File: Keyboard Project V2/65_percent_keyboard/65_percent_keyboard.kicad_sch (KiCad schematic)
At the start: 5 parts, among them U1 ATmega32A-P, Y1 16MHz

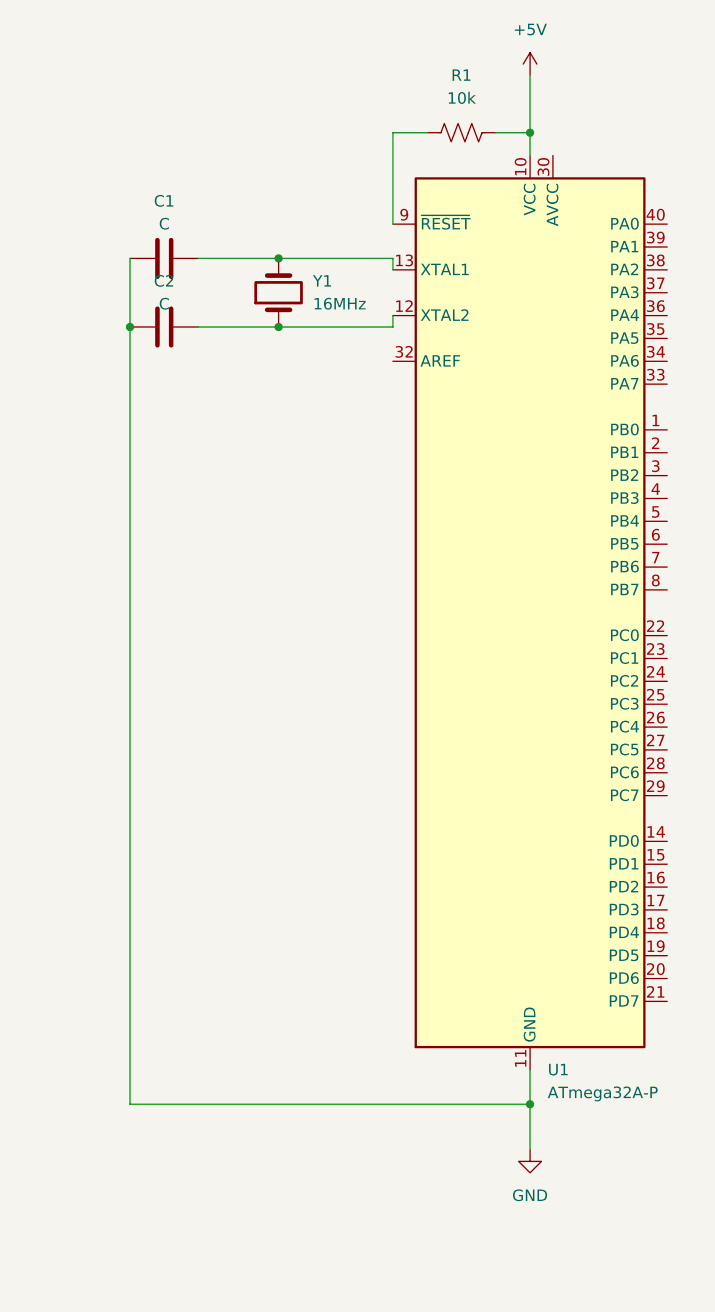
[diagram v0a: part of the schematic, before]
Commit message: updated directory
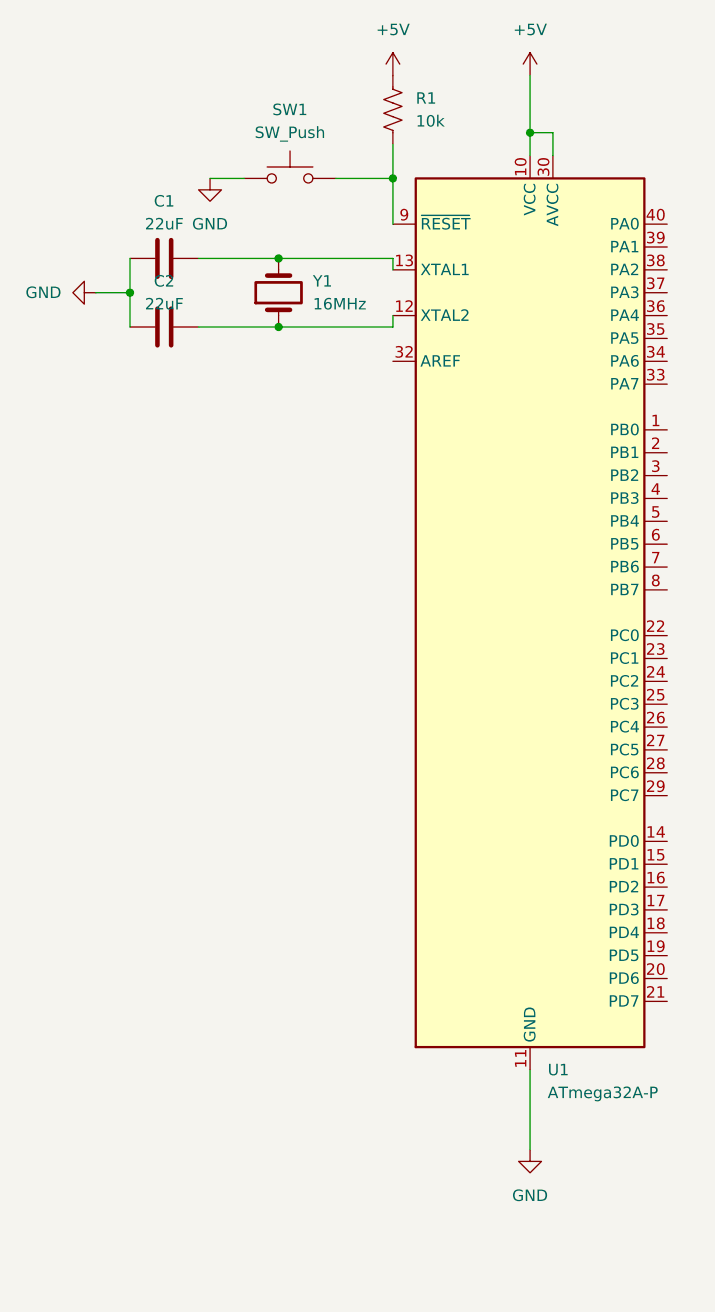
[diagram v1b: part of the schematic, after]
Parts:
- added SW1: SW_Push, symbol Switch:SW_Push
- C1, C2: value C -> 22uF
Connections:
- net +5V: now also U1.30 (AVCC)
- net GND: now also SW1.1
- net at R1.1, U1.9 (~{RESET}): now also SW1.2
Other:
- moved on the sheet: R1
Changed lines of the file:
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@@
 (kicad_sch (version 20230121) (generator eeschema)
   (paper "A4")
-  (junction (at 66.04 143.51) (diameter 0) (color 0 0 0 0)
+  (junction (at 50.8 40.64) (diameter 0) (color 0 0 0 0)
+  )
+  (junction (at 21.59 53.34) (diameter 0) (color 0 0 0 0)
   )
   (junction (at 38.1 57.15) (diameter 0) (color 0 0 0 0)
@@
   (junction (at 66.04 35.56) (diameter 0) (color 0 0 0 0)
   )
-  (junction (at 21.59 57.15) (diameter 0) (color 0 0 0 0)
-  )
   (junction (at 38.1 49.53) (diameter 0) (color 0 0 0 0)
   )
-  (wire (pts (xy 21.59 49.53) (xy 21.59 57.15))
-    (stroke (width 0) (type default))
-  )
-  (wire (pts (xy 66.04 143.51) (xy 21.59 143.51))
-    (stroke (width 0) (type default))
-  )
-  (wire (pts (xy 50.8 45.72) (xy 50.8 35.56))
-    (stroke (width 0) (type default))
-  )
-  (wire (pts (xy 62.23 35.56) (xy 66.04 35.56))
-    (stroke (width 0) (type default))
-  )
-  (wire (pts (xy 50.8 35.56) (xy 54.61 35.56))
-    (stroke (width 0) (type default))
-  )
-  (wire (pts (xy 66.04 139.7) (xy 66.04 143.51))
+  (wire (pts (xy 68.58 35.56) (xy 68.58 38.1))
+    (stroke (width 0) (type default))
+  )
+  (wire (pts (xy 21.59 49.53) (xy 21.59 53.34))
+    (stroke (width 0) (type default))
+  )
+  (wire (pts (xy 50.8 40.64) (xy 50.8 45.72))
+    (stroke (width 0) (type default))
+  )
+  (wire (pts (xy 17.78 53.34) (xy 21.59 53.34))
+    (stroke (width 0) (type default))
+  )
+  (wire (pts (xy 21.59 53.34) (xy 21.59 57.15))
+    (stroke (width 0) (type default))
+  )
+  (wire (pts (xy 66.04 35.56) (xy 68.58 35.56))
     (stroke (width 0) (type default))
   )
@@
     (stroke (width 0) (type default))
   )
+  (wire (pts (xy 44.45 40.64) (xy 50.8 40.64))
+    (stroke (width 0) (type default))
+  )
   (wire (pts (xy 66.04 35.56) (xy 66.04 38.1))
     (stroke (width 0) (type default))
   )
+  (wire (pts (xy 50.8 36.83) (xy 50.8 40.64))
+    (stroke (width 0) (type default))
+  )
   (wire (pts (xy 38.1 49.53) (xy 50.8 49.53))
     (stroke (width 0) (type default))
   )
-  (wire (pts (xy 66.04 143.51) (xy 66.04 148.59))
-    (stroke (width 0) (type default))
-  )
-  (wire (pts (xy 21.59 143.51) (xy 21.59 57.15))
+  (wire (pts (xy 66.04 139.7) (xy 66.04 148.59))
     (stroke (width 0) (type default))
   )
   (wire (pts (xy 66.04 29.21) (xy 66.04 35.56))
+    (stroke (width 0) (type default))
+  )
+  (wire (pts (xy 34.29 40.64) (xy 30.48 40.64))
     (stroke (width 0) (type default))
   )
@@
         (path "/317806f0-7832-447d-a362-c03f416f1932"
           (reference "Y1") (unit 1)
+        )
+      )
+    )
+  )
+  (symbol (lib_id "power:GND") (at 30.48 40.64 0) (unit 1)
+    (in_bom yes) (on_board yes) (dnp no) (fields_autoplaced)
+    (property "Reference" "#PWR05" (at 30.48 46.99 0)
+      (effects (font (size 1.27 1.27)) hide)
+    )
+    (property "Value" "GND" (at 30.48 45.72 0)
+      (effects (font (size 1.27 1.27)))
+    )
+    (property "Footprint" "" (at 30.48 40.64 0)
+      (effects (font (size 1.27 1.27)) hide)
+    )
+    (property "Datasheet" "" (at 30.48 40.64 0)
+      (effects (font (size 1.27 1.27)) hide)
+    )
+    (pin "1")
+    (instances
+      (project "65_percent_keyboard"
+        (path "/317806f0-7832-447d-a362-c03f416f1932"
+          (reference "#PWR05") (unit 1)
         )
       )
@@
       (effects (font (size 1.27 1.27)))
     )
-    (property "Value" "C" (at 25.4 54.61 90)
+    (property "Value" "22uF" (at 25.4 54.61 90)
       (effects (font (size 1.27 1.27)))
     )
@@
         (path "/317806f0-7832-447d-a362-c03f416f1932"
           (reference "C2") (unit 1)
+        )
+      )
+    )
+  )
+  (symbol (lib_id "Switch:SW_Push") (at 39.37 40.64 0) (unit 1)
+    (in_bom yes) (on_board yes) (dnp no) (fields_autoplaced)
+    (property "Reference" "SW1" (at 39.37 33.02 0)
+      (effects (font (size 1.27 1.27)))
+    )
+    (property "Value" "SW_Push" (at 39.37 35.56 0)
+      (effects (font (size 1.27 1.27)))
+    )
+    (property "Footprint" "" (at 39.37 35.56 0)
+      (effects (font (size 1.27 1.27)) hide)
+    )
+    (property "Datasheet" "~" (at 39.37 35.56 0)
+      (effects (font (size 1.27 1.27)) hide)
+    )
+    (pin "1")
+    (pin "2")
+    (instances
+      (project "65_percent_keyboard"
+        (path "/317806f0-7832-447d-a362-c03f416f1932"
+          (reference "SW1") (unit 1)
+        )
+      )
+    )
+  )
+  (symbol (lib_id "power:GND") (at 17.78 53.34 270) (unit 1)
+    (in_bom yes) (on_board yes) (dnp no) (fields_autoplaced)
+    (property "Reference" "#PWR03" (at 11.43 53.34 0)
+      (effects (font (size 1.27 1.27)) hide)
+    )
+    (property "Value" "GND" (at 13.97 53.34 90)
+      (effects (font (size 1.27 1.27)) (justify right))
+    )
+    (property "Footprint" "" (at 17.78 53.34 0)
+      (effects (font (size 1.27 1.27)) hide)
+    )
+    (property "Datasheet" "" (at 17.78 53.34 0)
+      (effects (font (size 1.27 1.27)) hide)
+    )
+    (pin "1")
+    (instances
+      (project "65_percent_keyboard"
+        (path "/317806f0-7832-447d-a362-c03f416f1932"
+          (reference "#PWR03") (unit 1)
         )
       )
@@
       (effects (font (size 1.27 1.27)))
     )
-    (property "Value" "C" (at 25.4 45.72 90)
+    (property "Value" "22uF" (at 25.4 45.72 90)
       (effects (font (size 1.27 1.27)))
     )
@@
     )
   )
+  (symbol (lib_id "power:+5V") (at 50.8 29.21 0) (unit 1)
+    (in_bom yes) (on_board yes) (dnp no) (fields_autoplaced)
+    (property "Reference" "#PWR04" (at 50.8 33.02 0)
+      (effects (font (size 1.27 1.27)) hide)
+    )
+    (property "Value" "+5V" (at 50.8 24.13 0)
+      (effects (font (size 1.27 1.27)))
+    )
+    (property "Footprint" "" (at 50.8 29.21 0)
+      (effects (font (size 1.27 1.27)) hide)
+    )
+    (property "Datasheet" "" (at 50.8 29.21 0)
+      (effects (font (size 1.27 1.27)) hide)
+    )
+    (pin "1")
+    (instances
+      (project "65_percent_keyboard"
+        (path "/317806f0-7832-447d-a362-c03f416f1932"
+          (reference "#PWR04") (unit 1)
+        )
+      )
+    )
+  )
   (symbol (lib_id "power:GND") (at 66.04 148.59 0) (unit 1)
     (in_bom yes) (on_board yes) (dnp no) (fields_autoplaced)
@@
     )
   )
-  (symbol (lib_id "Device:R_US") (at 58.42 35.56 90) (unit 1)
-    (in_bom yes) (on_board yes) (dnp no) (fields_autoplaced)
-    (property "Reference" "R1" (at 58.42 29.21 90)
-      (effects (font (size 1.27 1.27)))
-    )
-    (property "Value" "10k" (at 58.42 31.75 90)
-      (effects (font (size 1.27 1.27)))
-    )
-    (property "Footprint" "" (at 58.674 34.544 90)
-      (effects (font (size 1.27 1.27)) hide)
-    )
-    (property "Datasheet" "~" (at 58.42 35.56 0)
-      (effects (font (size 1.27 1.27)) hide)
-    )
+  (symbol (lib_id "Device:R_US") (at 50.8 33.02 180) (unit 1)
+    (in_bom yes) (on_board yes) (dnp no) (fields_autoplaced)
+    (property "Reference" "R1" (at 53.34 31.75 0)
+      (effects (font (size 1.27 1.27)) (justify right))
+    )
+    (property "Value" "10k" (at 53.34 34.29 0)
+      (effects (font (size 1.27 1.27)) (justify right))
+    )
+    (property "Footprint" "" (at 49.784 32.766 90)
+      (effects (font (size 1.27 1.27)) hide)
+    )
+    (property "Datasheet" "~" (at 50.8 33.02 0)
+      (effects (font (size 1.27 1.27)) hide)
+    )
